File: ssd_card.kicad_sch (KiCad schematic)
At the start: 6 parts, among them J1 SmartCard_ISO7816, Q1 2N7002, U1 STM32F405RGTx, U2 TPD4E05U06DQA

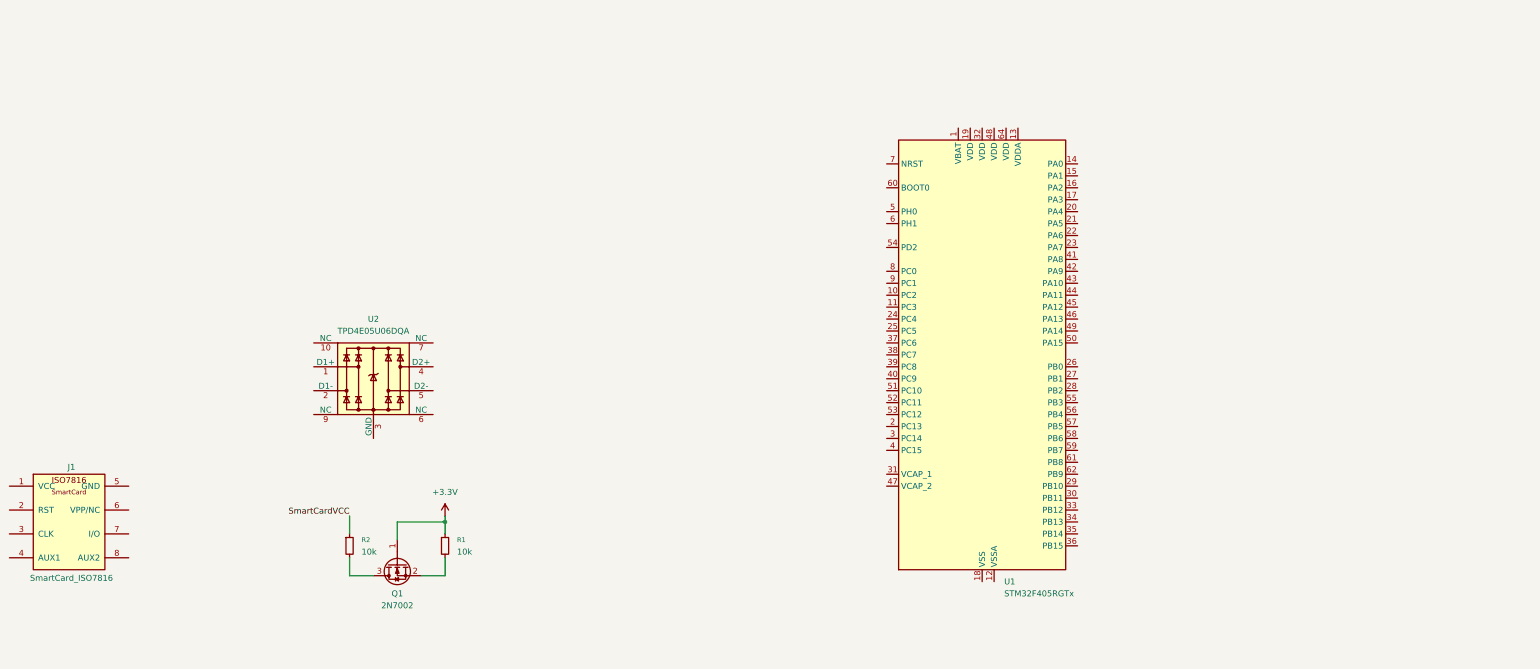
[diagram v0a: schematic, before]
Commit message: feat: Documentation
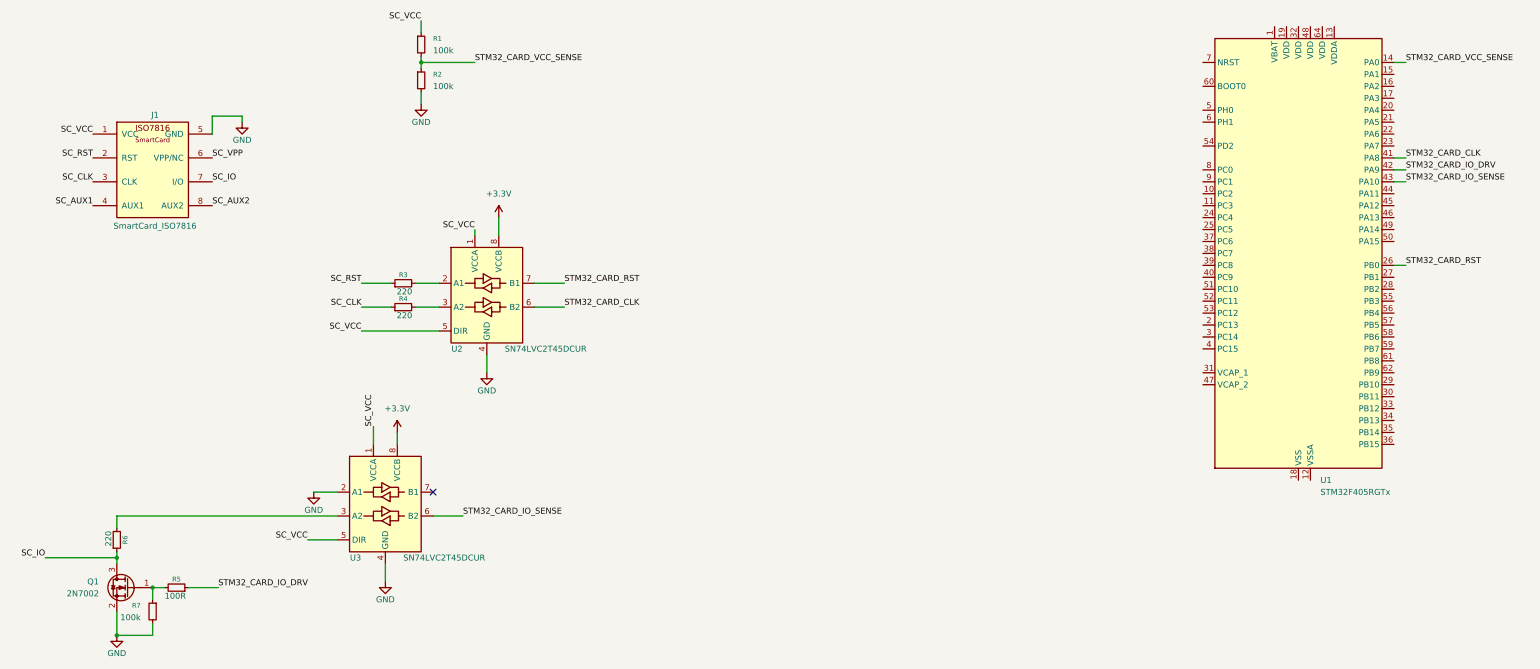
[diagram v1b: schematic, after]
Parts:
- removed U2: TPD4E05U06DQA, Package_SON:USON-10_2.5x1.0mm_P0.5mm, symbol Power_Protection:TPD4E05U06DQA
- added R3, R4, R6: 220, symbol Device:R_Small
- added R5: 100R, symbol Device:R_Small
- added R7: 100k, symbol Device:R_Small
- added U2, U3: SN74LVC2T45DCUR, Package_SO:VSSOP-8_2.3x2mm_P0.5mm, symbol Logic_LevelTranslator:SN74LVC2T45DCUR
- R1, R2: value 10k -> 100k
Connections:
- net SmartCardVCC is gone; now on net STM32_CARD_VCC_SENSE: R2.1
- net +3.3V: now also U2.8 (VCCB), U3.8 (VCCB); no longer Q1.1 (G), R1.1
- net SC_VCC: now reaches J1.1 (VCC)
- net SC_VCC: now also R1.1, U2.1 (VCCA), U2.5 (DIR), U3.1 (VCCA), U3.5 (DIR)
- net SC_RST: now reaches J1.2 (RST)
- net SC_RST: now also R3.1
- net SC_CLK: now reaches J1.3 (CLK)
- net SC_CLK: now also R4.1
- net SC_AUX1: now reaches J1.4 (AUX1)
- net GND: now reaches J1.5 (GND)
- net GND: now also Q1.2 (S), R2.2, R7.2, U2.4 (GND), U3.2 (A1), U3.4 (GND)
- net SC_VPP: now reaches J1.6 (VPP/NC)
- net SC_IO: now reaches J1.7 (I/O)
- net SC_IO: now also Q1.3 (D), R6.1
- net SC_AUX2: now reaches J1.8 (AUX2)
- net STM32_CARD_VCC_SENSE: now reaches R1.2
- net STM32_CARD_VCC_SENSE: now also U1.14 (PA0); no longer Q1.2 (S)
- net STM32_CARD_RST: now reaches U1.26 (PB0)
- net STM32_CARD_RST: now also U2.7 (B1)
- net STM32_CARD_CLK: now reaches U1.41 (PA8)
- net STM32_CARD_CLK: now also U2.6 (B2)
- net STM32_CARD_IO_DRV: now reaches U1.42 (PA9)
- net STM32_CARD_IO_DRV: now also R5.1
- net STM32_CARD_IO_SENSE: now reaches U1.43 (PA10)
- net STM32_CARD_IO_SENSE: now also U3.6 (B2)
- new net: R4.2, U2.3 (A2)
- new net: Q1.1 (G), R5.2, R7.1
- new net: R3.2, U2.2 (A1)
- new net: R6.2, U3.3 (A2)
- no-connect marks 0 -> 1
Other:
- moved on the sheet: J1, U1
